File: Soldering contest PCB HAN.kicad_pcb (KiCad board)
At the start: 2 copper layers, 99.1 x 98.6 mm, 18 parts, among them J1 Screw_Terminal_01x02, Q1 2N3904, Q2 2N3904

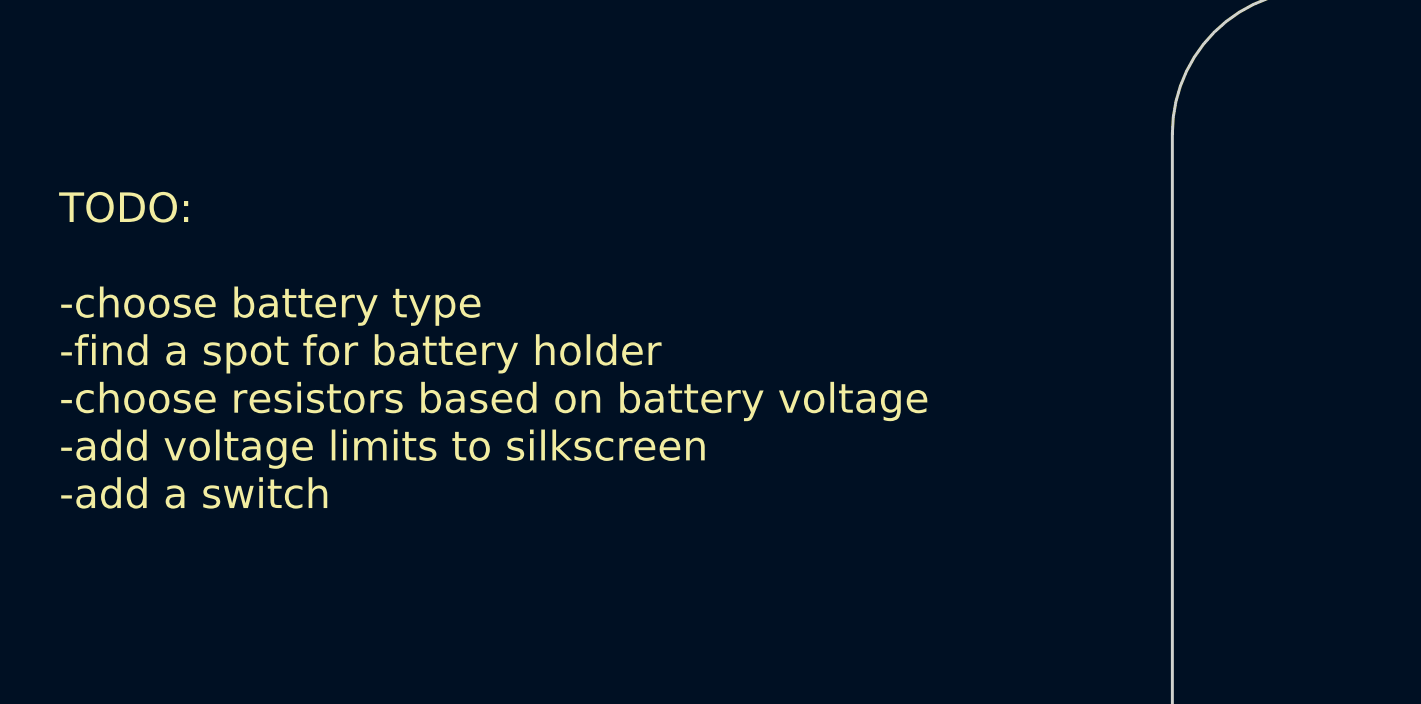
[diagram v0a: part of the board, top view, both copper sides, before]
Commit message: Working on ERC
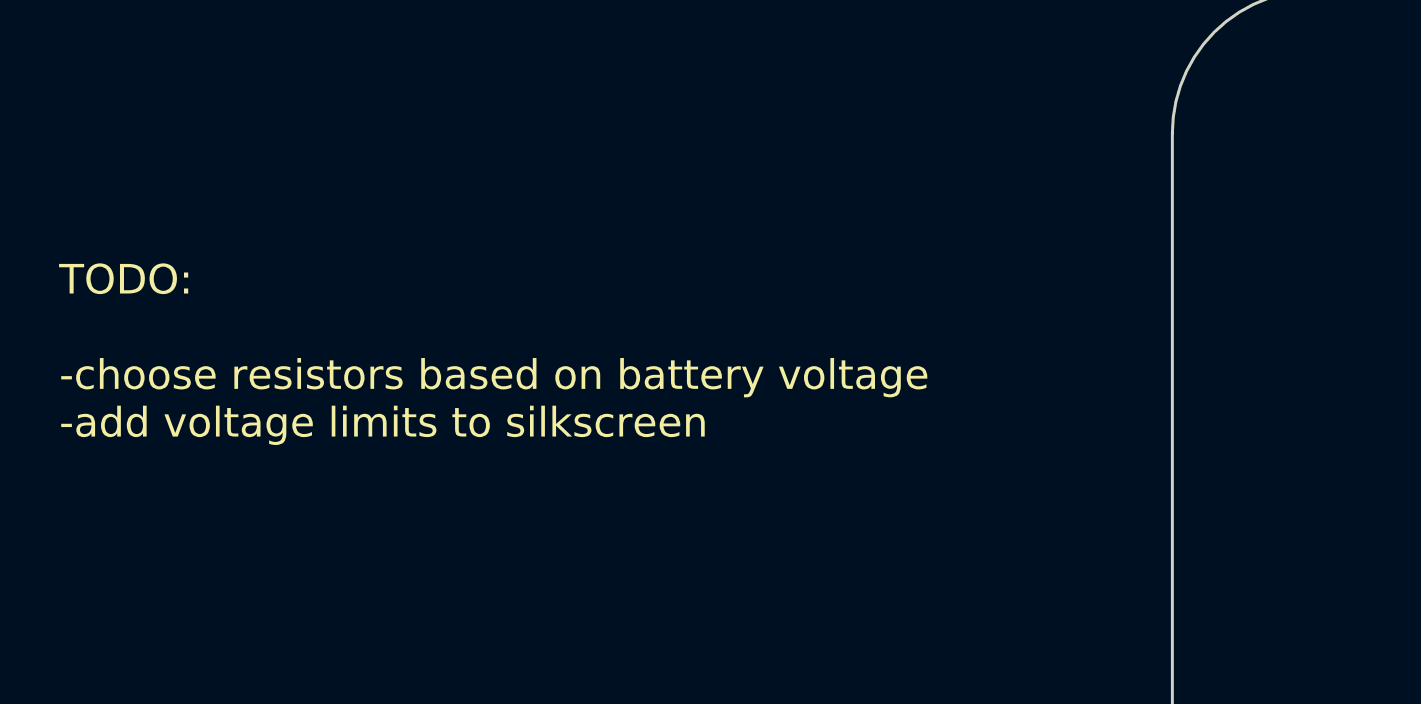
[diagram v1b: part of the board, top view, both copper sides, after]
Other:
- board text added: "TODO: -choose resistors based on battery voltage -add voltage limits to silkscreen"
- board text removed: "TODO: -choose battery type -find a spot for battery holder -choose resistors based on battery voltage -add voltage limits to silkscreen -add a switch"
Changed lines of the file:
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@@
     (effects (font (size 1 1) (thickness 0.15)))
   )
-  (gr_text "TODO:\n\n-choose battery type\n-find a spot for battery holder\n-choose resistors based on battery voltage\n-add voltage limits to silkscreen\n-add a switch" (at 73.66 63.5) (layer "F.SilkS")
+  (gr_text "TODO:\n\n-choose resistors based on battery voltage\n-add voltage limits to silkscreen\n" (at 73.66 63.5) (layer "F.SilkS")
     (effects (font (size 1 1) (thickness 0.15)) (justify left))
   )
